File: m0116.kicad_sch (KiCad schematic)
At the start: 247 parts, among them J2 Conn_01x04_MountingPin, J3 Conn_01x04_MountingPin, Q1 Q_PMOS_GSD AO3401A, Q2 Q_NMOS_GSD 2N7002, Q3 Q_NMOS_GSD 2N7002, Q4 2N3904, SW1 SW_Push, U1 XC6206P332MR, U2 74AHCT1G125, U3 STM32F411RETx, U4 24LC64, U5 USBLC6-2SC6, Y1 8MHz

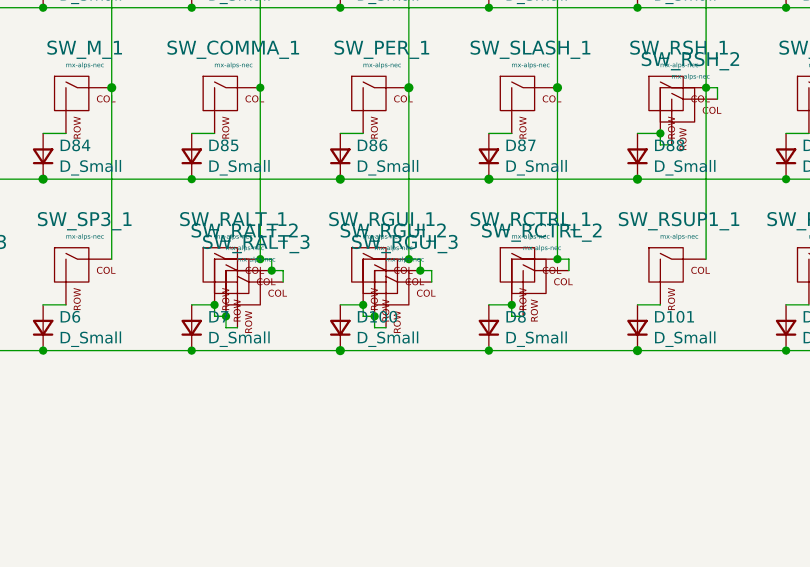
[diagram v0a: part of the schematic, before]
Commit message: updates
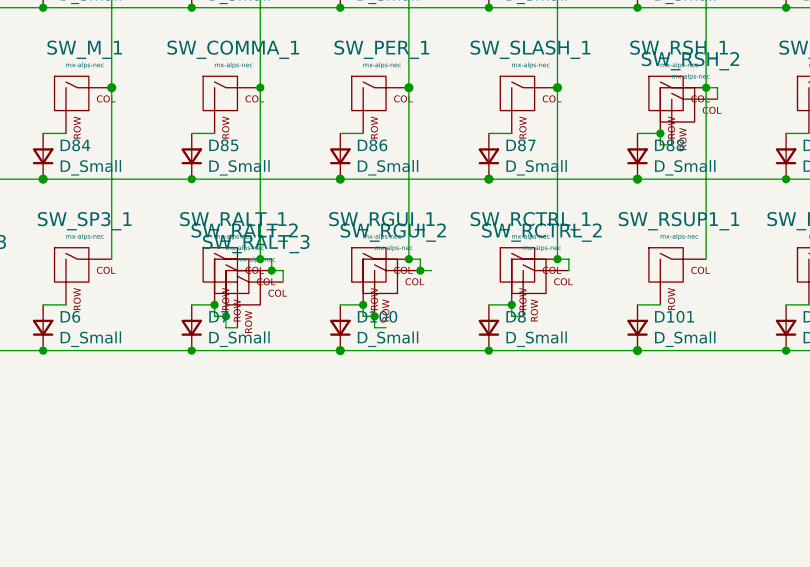
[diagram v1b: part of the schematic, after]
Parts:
- removed SW_RGUI_3: mx-alps-nec, Alps_Only:ALPS-1U, symbol MX_Alps_Hybrid:mx-alps-nec
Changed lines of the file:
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@@
     (stroke (width 0) (type default))
   )
-  (wire (pts (xy 186.69 344.17) (xy 186.69 345.44))
-    (stroke (width 0) (type default))
-  )
   (wire (pts (xy 193.04 309.88) (xy 195.58 309.88))
     (stroke (width 0) (type solid))
@@
         )
       )
-    )
-  )
-  (symbol (lib_id "MX_Alps_Hybrid:mx-alps-nec") (at 182.88 346.71 0) (unit 1)
-    (in_bom yes) (on_board yes) (dnp no)
-    (property "Reference" "SW_RGUI_3" (at 183.7182 341.0458 0)
-      (effects (font (size 1.524 1.524)))
-    )
-    (property "Value" "mx-alps-nec" (at 183.7182 342.9254 0)
-      (effects (font (size 0.508 0.508)))
-    )
-    (property "Footprint" "Alps_Only:ALPS-1U" (at 167.005 347.345 0)
-      (effects (font (size 1.524 1.524)) hide)
-    )
-    (property "Datasheet" "" (at 167.005 347.345 0)
-      (effects (font (size 1.524 1.524)) hide)
-    )
-    (pin "1")
-    (pin "2")
-    (instances
-      (project "m0116"
-        (path "/151da08b-0979-4785-a9bf-6fa9b165d629"
-          (reference "SW_RGUI_3") (unit 1)
-        )
-      )

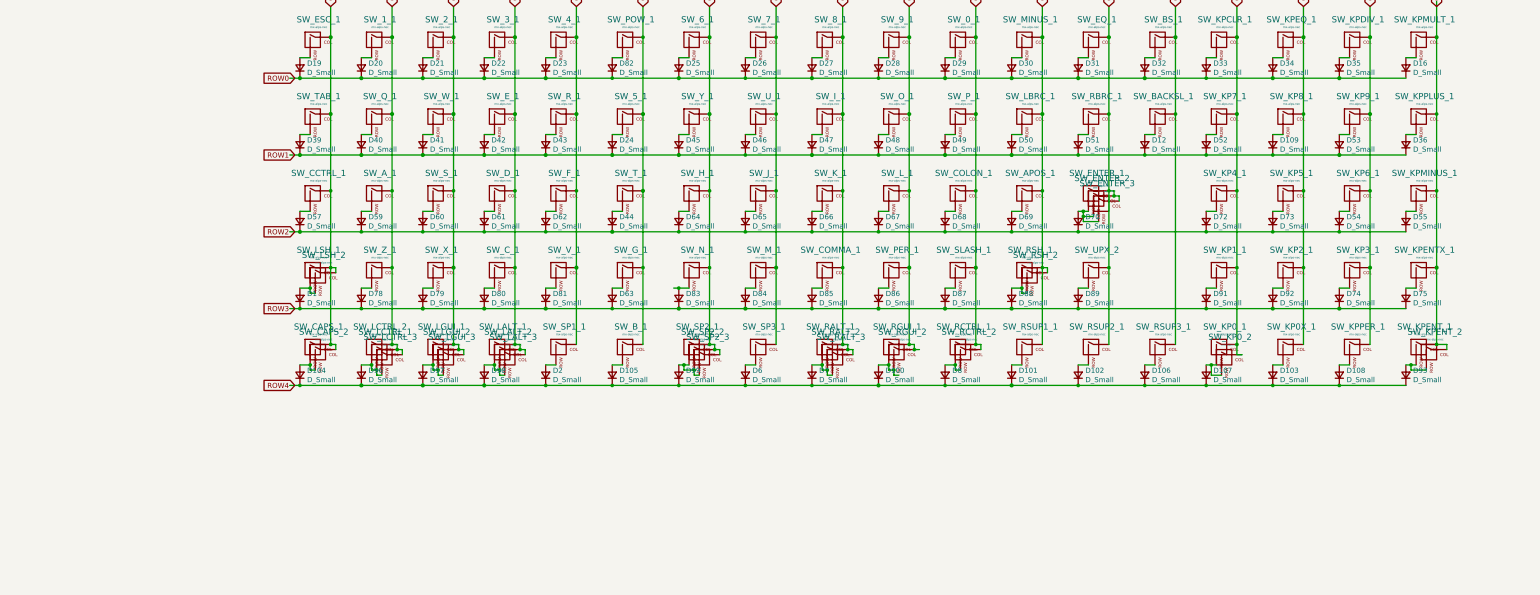
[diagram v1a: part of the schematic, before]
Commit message: fixes
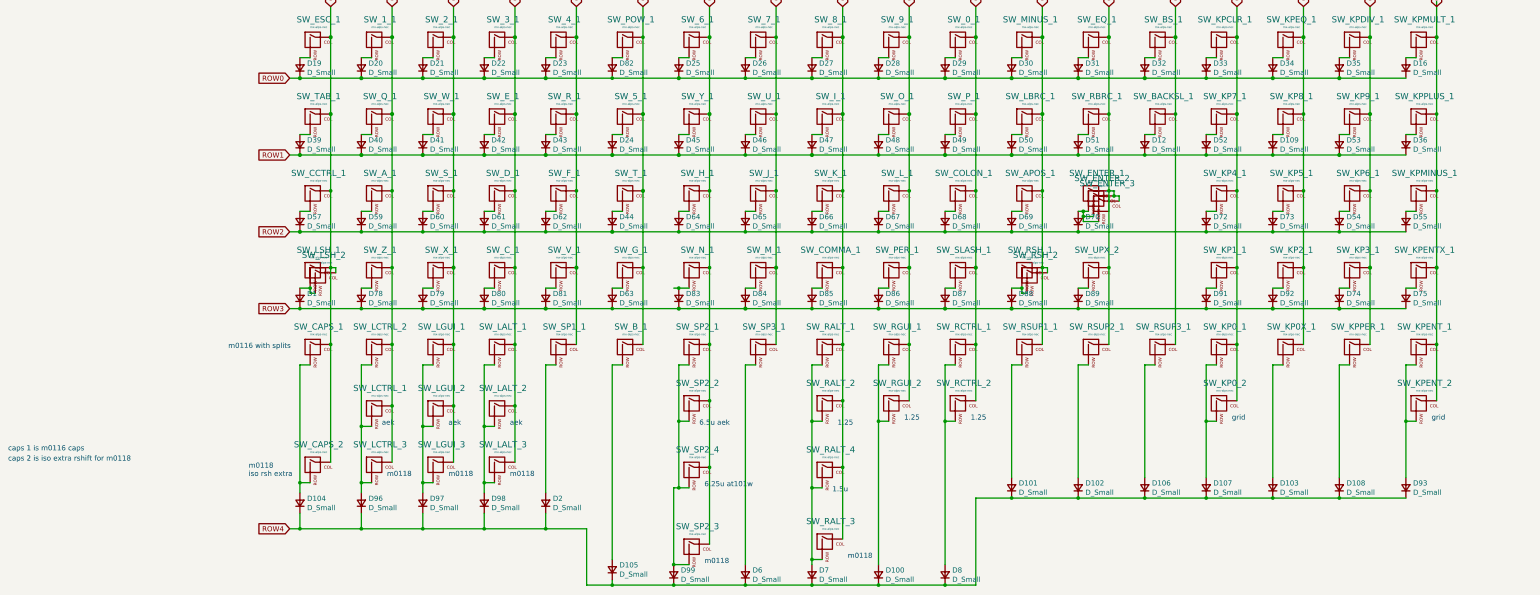
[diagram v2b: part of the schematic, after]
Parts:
- added SW_RALT_4, SW_SP2_4: mx-alps-nec, Alps_Only:ALPS-1U, symbol MX_Alps_Hybrid:mx-alps-nec
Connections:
- net COL6: now also SW_SP2_4.1 (COL)
- net COL8: now also SW_RALT_4.1 (COL)
- net at D7.2 (A), SW_RALT_1.2 (ROW), SW_RALT_2.2 (ROW)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: now also SW_RALT_4.2 (ROW)
- net at D99.2 (A), SW_SP2_1.2 (ROW), SW_SP2_2.2 (ROW)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: now also SW_SP2_4.2 (ROW)
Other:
- note added: "1.25"
- note added: "1.5u"
- note added: "6.25u at101w"
- note added: "6.5u aek"
- note added: "aek"
- note added: "caps 1 is m0116 caps"
- note added: "caps 2 is iso extra rshift for m0118"
- note added: "grid"
- note added: "m0116 with splits"
- note added: "m0118"
- note added: "m0118 iso rsh extra"
- moved on the sheet: D100, D101, D102, D103, D104, D105, D106, D107, D108, D2, D6, D7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
